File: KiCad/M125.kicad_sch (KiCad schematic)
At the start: 20 parts, among them J1 Conn_01x04, J2 Conn_01x04, J3 Shelly, Q1 PMF250XNEX, U1 ESP32-PICO-MINI-02, U2 LMR16006+FB

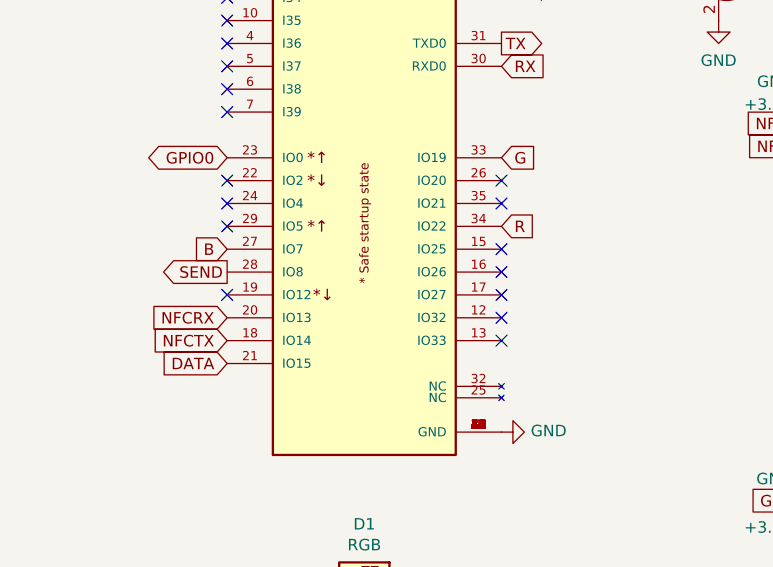
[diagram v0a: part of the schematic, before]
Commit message: New PCB
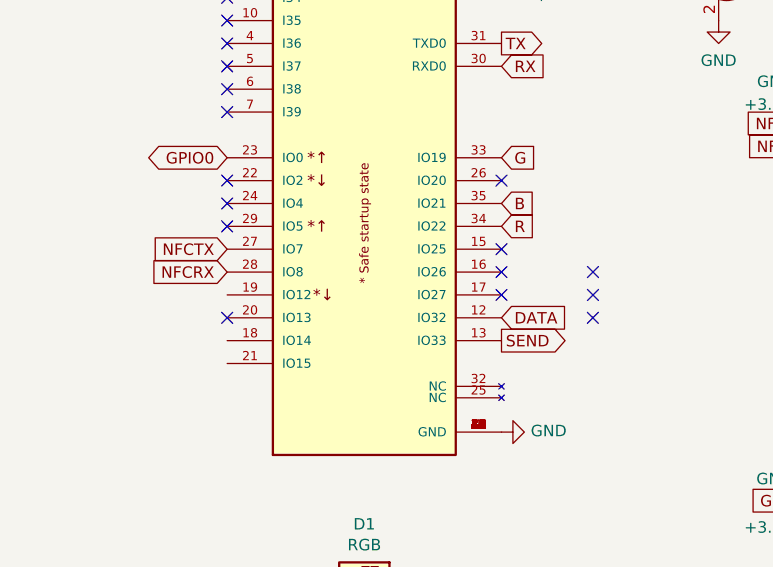
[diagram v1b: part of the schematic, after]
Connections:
- net B: now also U1.35 (IO21); no longer U1.27 (IO7)
- net DATA: now also U1.12 (IO32); no longer U1.21 (IO15)
- net NFCRX: now also U1.28 (IO8); no longer U1.20 (IO13)
- net NFCTX: now also U1.27 (IO7); no longer U1.18 (IO14)
- net SEND: now also U1.13 (IO33); no longer U1.28 (IO8)
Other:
- title: Generic ESP32-PICO-MINI module -> M-125 control
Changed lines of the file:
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@@
   (paper "A4")
   (title_block
-    (title "Generic ESP32-PICO-MINI module")
+    (title "M-125 control")
     (date "${DATE}")
     (rev "1")
@@
   (no_connect (at 50.8 66.04))
   (no_connect (at 50.8 71.12))
-  (no_connect (at 50.8 78.74))
-  (no_connect (at 81.28 68.58))
-  (no_connect (at 81.28 81.28))
-  (no_connect (at 81.28 83.82))
+  (no_connect (at 50.8 81.28))
+  (no_connect (at 91.44 76.2))
+  (no_connect (at 91.44 78.74))
+  (no_connect (at 91.44 81.28))
   (wire (pts (xy 220.98 38.1) (xy 231.775 38.1))
     (stroke (width 0) (type default) (color 0 0 0 0))
@@
     )
   )
-  (global_label "NFCRX" (shape input) (at 50.8 81.28 180) (fields_autoplaced)
-    (effects (font (size 1.27 1.27)) (justify right))
-    (property "Intersheet References" "${INTERSHEET_REFS}" (id 0) (at 42.3072 81.2006 0)
+  (global_label "NFCRX" (shape input) (at 50.8 76.2 180) (fields_autoplaced)
+    (effects (font (size 1.27 1.27)) (justify right))
+    (property "Intersheet References" "${INTERSHEET_REFS}" (id 0) (at 42.3072 76.1206 0)
       (effects (font (size 1.27 1.27)) (justify right) hide)
     )
@@
     )
   )
-  (global_label "SEND" (shape output) (at 50.8 76.2 180) (fields_autoplaced)
-    (effects (font (size 1.27 1.27)) (justify right))
-    (property "Intersheet References" "${INTERSHEET_REFS}" (id 0) (at 43.5168 76.1206 0)
-      (effects (font (size 1.27 1.27)) (justify right) hide)
+  (global_label "SEND" (shape output) (at 81.28 83.82 0) (fields_autoplaced)
+    (effects (font (size 1.27 1.27)) (justify left))
+    (property "Intersheet References" "${INTERSHEET_REFS}" (id 0) (at 88.5632 83.8994 0)
+      (effects (font (size 1.27 1.27)) (justify left) hide)
     )
   )
@@
     )
   )
-  (global_label "DATA" (shape input) (at 50.8 86.36 180) (fields_autoplaced)
-    (effects (font (size 1.27 1.27)) (justify right))
-    (property "Intersheet References" "${INTERSHEET_REFS}" (id 0) (at 44.061 86.2806 0)
-      (effects (font (size 1.27 1.27)) (justify right) hide)
+  (global_label "DATA" (shape input) (at 81.28 81.28 0) (fields_autoplaced)
+    (effects (font (size 1.27 1.27)) (justify left))
+    (property "Intersheet References" "${INTERSHEET_REFS}" (id 0) (at 88.019 81.3594 0)
+      (effects (font (size 1.27 1.27)) (justify left) hide)
     )
   )
@@
     )
   )
-  (global_label "NFCTX" (shape input) (at 50.8 83.82 180) (fields_autoplaced)
-    (effects (font (size 1.27 1.27)) (justify right))
-    (property "Intersheet References" "${INTERSHEET_REFS}" (id 0) (at 42.6096 83.7406 0)
+  (global_label "NFCTX" (shape input) (at 50.8 73.66 180) (fields_autoplaced)
+    (effects (font (size 1.27 1.27)) (justify right))
+    (property "Intersheet References" "${INTERSHEET_REFS}" (id 0) (at 42.6096 73.5806 0)
       (effects (font (size 1.27 1.27)) (justify right) hide)
     )
@@
     )
   )
-  (global_label "B" (shape input) (at 50.8 73.66 180) (fields_autoplaced)
-    (effects (font (size 1.27 1.27)) (justify right))
-    (property "Intersheet References" "${INTERSHEET_REFS}" (id 0) (at -52.07 -31.75 0)
-      (effects (font (size 1.27 1.27)) hide)
-    )
+  (global_label "B" (shape input) (at 81.28 68.58 0) (fields_autoplaced)
+    (effects (font (size 1.27 1.27)) (justify left))
+    (property "Intersheet References" "${INTERSHEET_REFS}" (id 0) (at 184.15 173.99 0)
+      (effects (font (size 1.27 1.27)) hide)
+    )
